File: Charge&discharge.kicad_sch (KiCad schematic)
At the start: 117 parts, among them Q1 NMOS, Q10 NMOS, Q11 NMOS, Q12 NMOS, Q13 NMOS, Q14 NMOS, Q15 NMOS, Q16 NMOS, Q17 NMOS, Q18 NMOS, Q19 NMOS, Q2 NMOS, Q20 NMOS, Q21 NMOS, Q22 NMOS, Q23 NMOS, Q24 NMOS, Q25 NMOS, Q26 NMOS, Q27 NMOS, Q28 NMOS, Q29 NMOS, Q3 NMOS, Q30 NMOS, Q31 NMOS, Q32 NMOS, Q33 NMOS, Q34 NMOS, Q35 NMOS, Q36 NMOS, Q37 NMOS, Q38 NMOS, Q39 NMOS, Q4 NMOS, Q40 NMOS, Q41 NPN, Q5 NMOS, Q6 NMOS, Q62 NPN, Q63 NPN, Q64 NPN, Q65 NPN, Q66 NMOS, Q7 NMOS, Q8 NMOS, Q9 NMOS, U10 SFH617A-1, U11 SFH617A-1, U12 BZT52C16_C2903915, U13 BZT52C16_C2903915, U8 SFH617A-1, U9 SFH617A-1

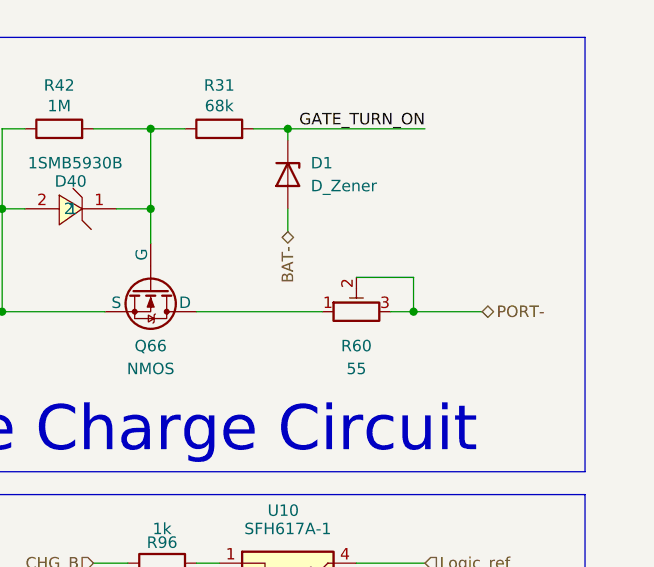
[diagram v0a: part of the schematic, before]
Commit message: MVP Friday
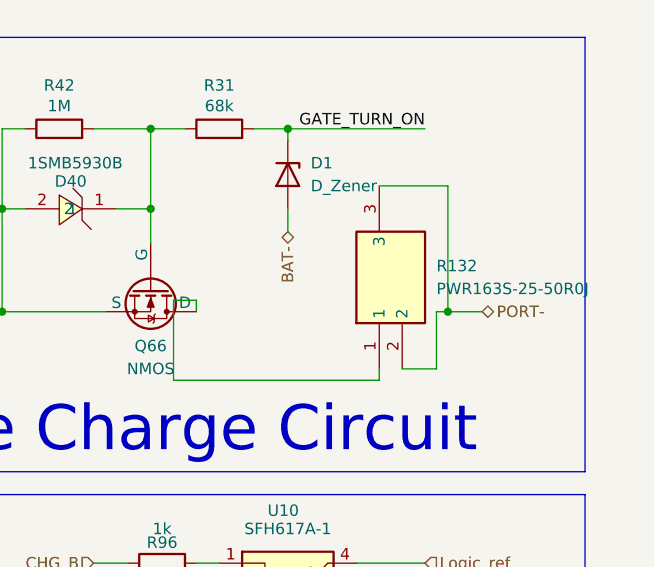
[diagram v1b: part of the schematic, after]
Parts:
- removed R60: 55, symbol Device:R_Potentiometer_Trim
- added R132: PWR163S-25-50R0J, PWR163S-25-50R0J:PWR163S2550R0F, symbol PWR136S-25-50R0J:PWR163S-25-50R0J
- R1, R10, R11, R12, R13, R14, R15, R16, R17, R18, R19, R2, R20, R21, R22, R23, R24, R25, R26, R27, R28, R29, R3, R30, R32, R33, R34, R35, R36, R37, R38, R39, R4, R40, R41, R5, R6, R7, R8, R9: footprint (none) -> Resistor_SMD:R_0201_0603Metric; LCSC (none) -> C7467289
- R31: footprint (none) -> Resistor_SMD:R_0805_2012Metric; LCSC (none) -> C407437
- R42: footprint (none) -> Resistor_SMD:R_0805_2012Metric; LCSC (none) -> C2771009
- R43: footprint (none) -> Resistor_SMD:R_2512_6332Metric; LCSC (none) -> C22383486
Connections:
- net PORT-: now also R132.2, R132.3
- net at Q66.1 (D): now also R132.1
